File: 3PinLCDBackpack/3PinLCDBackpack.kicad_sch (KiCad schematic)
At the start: 7 parts, among them Q1 BC547, U1 74HC595, U2 LCD_HD44780, U3 5-pin_LiquidCrystal595_connec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

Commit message: 3-pin
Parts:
- U2: footprint My_Parts:LCD_HD44780_16x2_w_headers_large -> My_Parts:LCD_HD44780_16x2_w_headers_no outlinelarge
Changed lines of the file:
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@@
       (effects (font (size 1.27 1.27)) (justify left))
     )
-    (property "Footprint" "My_Parts:LCD_HD44780_16x2_w_headers_large" (id 2) (at 203.2 121.92 0)
+    (property "Footprint" "My_Parts:LCD_HD44780_16x2_w_headers_no outlinelarge" (id 2) (at 203.2 121.92 0)
       (effects (font (size 1.27 1.27)) hide)
     )
@@
     )
     (path "/00000000-0000-0000-0000-000061513e75"
-      (reference "U2") (unit 1) (value "LCD_HD44780") (footprint "My_Parts:LCD_HD44780_16x2_w_headers_large")
+      (reference "U2") (unit 1) (value "LCD_HD44780") (footprint "My_Parts:LCD_HD44780_16x2_w_headers_no outlinelarge")
     )
     (path "/aabd25b2-274f-420f-b1ab-3c5ed40de82c"

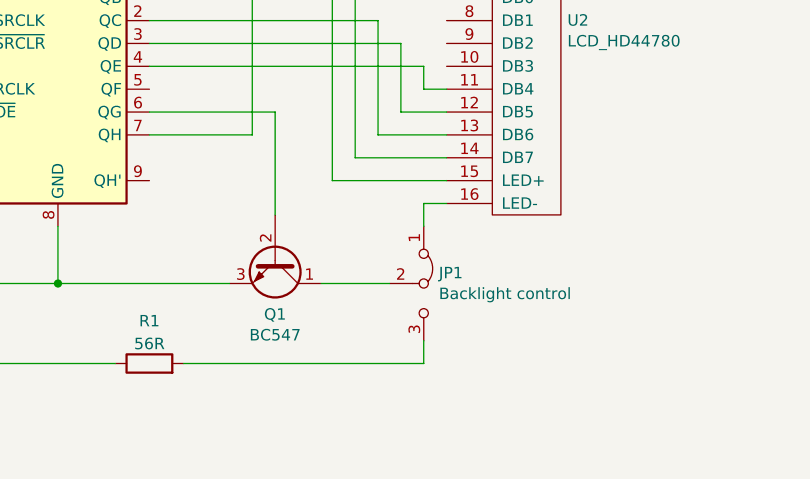
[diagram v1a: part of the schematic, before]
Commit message: 3pinLCD
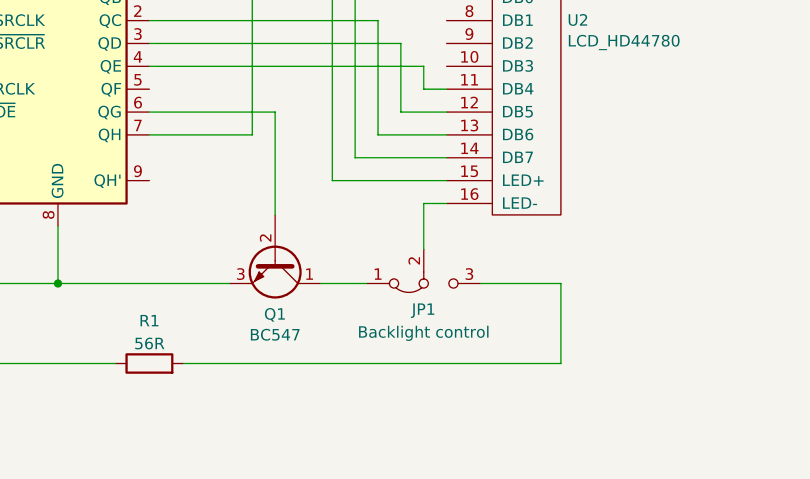
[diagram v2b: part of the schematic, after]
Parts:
- removed JP1: Backlight control, My_Parts:Jumper_1x03_P2.54mm_large, symbol 3PinLCDBackpack-rescue:Jumper_3_Bridged12-Jumper
- added JP1: Backlight control, My_Parts:Angled_Jumper_1x03_P2.54mm_large, symbol Jumper:Jumper_3_Bridged12
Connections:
- net at U2.16 (LED-): now also JP1.2 (C)
- net at Q1.1 (C): now also JP1.1 (A)
- net at R1.2: now also JP1.3 (B)
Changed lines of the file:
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@@
+    (stroke (width 0) (type default) (color 0 0 0 0))
+  )
+  (wire (pts (xy 189.23 134.62) (xy 189.23 125.73))
     (stroke (width 0) (type default) (color 0 0 0 0))
   )
@@
     (stroke (width 0) (type default) (color 0 0 0 0))
   )
+  (wire (pts (xy 189.23 125.73) (xy 180.34 125.73))
+    (stroke (width 0) (type default) (color 0 0 0 0))
+  )
   (wire (pts (xy 113.03 69.85) (xy 113.03 104.14))
     (stroke (width 0) (type default) (color 0 0 0 0))
@@
     (stroke (width 0) (type default) (color 0 0 0 0))
   )
+  (wire (pts (xy 162.56 125.73) (xy 167.64 125.73))
+    (stroke (width 0) (type default) (color 0 0 0 0))
+  )
   (wire (pts (xy 118.11 67.31) (xy 118.11 91.44))
     (stroke (width 0) (type default) (color 0 0 0 0))
@@
     (stroke (width 0) (type default) (color 0 0 0 0))
   )
-  (wire (pts (xy 170.18 125.73) (xy 162.56 125.73))
-    (stroke (width 0) (type default) (color 0 0 0 0))
-  )
   (wire (pts (xy 176.53 83.82) (xy 154.94 83.82))
     (stroke (width 0) (type default) (color 0 0 0 0))
@@
     (stroke (width 0) (type default) (color 0 0 0 0))
   )
-  (wire (pts (xy 173.99 119.38) (xy 173.99 116.84))
-    (stroke (width 0) (type default) (color 0 0 0 0))
-  )
-  (wire (pts (xy 173.99 132.08) (xy 173.99 134.62))
+  (wire (pts (xy 173.99 116.84) (xy 173.99 121.92))
     (stroke (width 0) (type default) (color 0 0 0 0))
   )
@@
     (stroke (width 0) (type default) (color 0 0 0 0))
   )
-  (wire (pts (xy 147.32 134.62) (xy 173.99 134.62))
+  (wire (pts (xy 147.32 134.62) (xy 189.23 134.62))
     (stroke (width 0) (type default) (color 0 0 0 0))
   )
@@
     (pin "3")
   )
-  (symbol (lib_id "3PinLCDBackpack-rescue:Jumper_3_Bridged12-Jumper") (at 173.99 125.73 270) (unit 1)
-    (in_bom yes) (on_board yes)
-    (property "Reference" "JP1" (id 0) (at 175.6664 124.5616 90)
-      (effects (font (size 1.27 1.27)) (justify left))
-    )
-    (property "Value" "Backlight control" (id 1) (at 175.6664 126.873 90)
-      (effects (font (size 1.27 1.27)) (justify left))
-    )
-    (property "Footprint" "My_Parts:Jumper_1x03_P2.54mm_large" (id 2) (at 173.99 125.73 0)
+  (symbol (lib_id "Jumper:Jumper_3_Bridged12") (at 173.99 125.73 0) (mirror x) (unit 1)
+    (in_bom yes) (on_board yes) (fields_autoplaced)
+    (property "Reference" "JP1" (id 0) (at 173.99 128.6246 0))
+    (property "Value" "Backlight control" (id 1) (at 173.99 131.1615 0))
+    (property "Footprint" "My_Parts:Angled_Jumper_1x03_P2.54mm_large" (id 2) (at 173.99 125.73 0)
       (effects (font (size 1.27 1.27)) hide)
     )
@@
       (reference "#PWR0102") (unit 1) (value "VCC") (footprint "")
     )
-    (path "/00000000-0000-0000-0000-000061564bcc"
-      (reference "JP1") (unit 1) (value "Backlight control") (footprint "My_Parts:Jumper_1x03_P2.54mm_large")
+    (path "/12393de5-06b2-4f3c-9de5-f3a24d04b4a0"
+      (reference "JP1") (unit 1) (value "Backlight control") (footprint "My_Parts:Angled_Jumper_1x03_P2.54mm_large")
     )
     (path "/00000000-0000-0000-0000-000061518afb"
